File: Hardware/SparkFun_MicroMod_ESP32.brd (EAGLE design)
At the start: 22 x 22 mm, 53 parts, among them J1 MICROMOD-2222, Q2 MBT3904DW1T1, U1 W25QXX128MBIT-6X5, U2 ESP3212, U4 CP2102N, Y1 40MHZ, Y2 32.768kHz

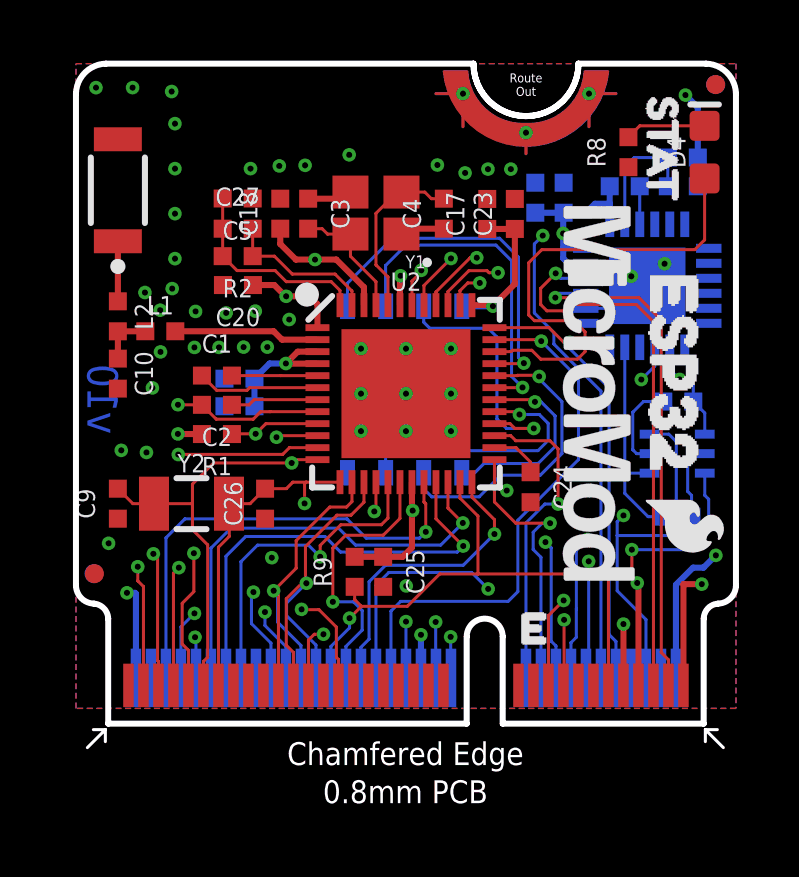
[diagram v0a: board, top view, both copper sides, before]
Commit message: Update SparkFun_MicroMod_ESP32.brd
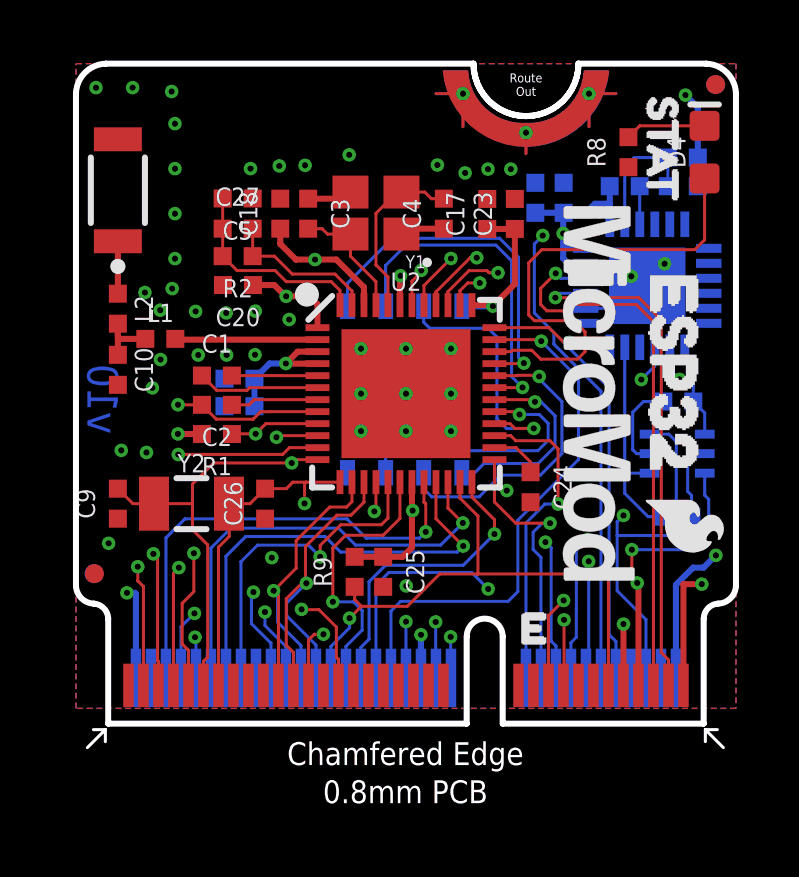
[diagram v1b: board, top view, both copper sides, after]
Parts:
- moved L2 0.25 mm to (1.40, 13.8)
- moved L1 0.25 mm to (2.81, 12.8)
- moved C10 0.13 mm to (1.40, 11.8)
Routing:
- net N$6: track 1.83 -> 2.44 mm
- net GND: vias 46 -> 45
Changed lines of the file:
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@@
 <?xml version="1.0" encoding="utf-8"?>
 <!DOCTYPE eagle SYSTEM "eagle.dtd">
-<eagle version="9.4.1">
+<eagle version="9.6.0">
 <drawing>
 <settings>
@@
 <setting verticaltext="up"/>
 </settings>
-<grid distance="0.05" unitdist="inch" unit="mm" style="lines" multiple="1" display="yes" altdistance="0.005" altunitdist="inch" altunit="inch"/>
+<grid distance="0.05" unitdist="inch" unit="inch" style="lines" multiple="1" display="yes" altdistance="0.005" altunitdist="inch" altunit="inch"/>
 <layers>
 <layer number="1" name="Top" color="4" fill="1" visible="yes" active="yes"/>
@@
 <layer number="38" name="bTest" color="7" fill="1" visible="no" active="yes"/>
 <layer number="39" name="tKeepout" color="4" fill="11" visible="yes" active="yes"/>
-<layer number="40" name="bKeepout" color="1" fill="11" visible="yes" active="yes"/>
+<layer number="40" name="bKeepout" color="1" fill="11" visible="no" active="yes"/>
 <layer number="41" name="tRestrict" color="4" fill="10" visible="no" active="yes"/>
 <layer number="42" name="bRestrict" color="1" fill="10" visible="no" active="yes"/>
 <layer number="43" name="vRestrict" color="2" fill="10" visible="no" active="yes"/>
 <layer number="44" name="Drills" color="7" fill="1" visible="no" active="yes"/>
-<layer number="45" name="Holes" color="7" fill="1" visible="no" active="yes"/>
+<layer number="45" name="Holes" color="7" fill="1" visible="yes" active="yes"/>
 <layer number="46" name="Milling" color="3" fill="1" visible="no" active="yes"/>
 <layer number="47" name="Measures" color="7" fill="1" visible="no" active="yes"/>
@@
 <layer number="50" name="dxf" color="7" fill="1" visible="no" active="yes"/>
 <layer number="51" name="tDocu" color="6" fill="1" visible="yes" active="yes"/>
-<layer number="52" name="bDocu" color="7" fill="1" visible="yes" active="yes"/>
+<layer number="52" name="bDocu" color="7" fill="1" visible="no" active="yes"/>
 <layer number="91" name="Nets" color="2" fill="1" visible="no" active="no"/>
 <layer number="92" name="Busses" color="1" fill="1" visible="no" active="no"/>
@@
 <layer number="95" name="Names" color="7" fill="1" visible="no" active="no"/>
 <layer number="96" name="Values" color="7" fill="1" visible="no" active="no"/>
-<layer number="2" name="Horz/PWR" color="16" fill="1" visible="yes" active="yes"/>
+<layer number="2" name="Horz/PWR" color="16" fill="1" visible="no" active="yes"/>
 <layer number="3" name="Route3" color="17" fill="1" visible="no" active="no"/>
 <layer number="4" name="Route4" color="18" fill="1" visible="no" active="no"/>
@@
 <layer number="13" name="Route13" color="21" fill="1" visible="no" active="no"/>
 <layer number="14" name="Route14" color="22" fill="1" visible="no" active="no"/>
-<layer number="15" name="VIRT/GND" color="23" fill="1" visible="yes" active="yes"/>
+<layer number="15" name="VIRT/GND" color="23" fill="1" visible="no" active="yes"/>
 <layer number="53" name="tGND_GNDA" color="7" fill="9" visible="no" active="no"/>
 <layer number="54" name="bGND_GNDA" color="1" fill="9" visible="no" active="no"/>
@@
 <attribute name="VALUE" x="7.781" y="11.137" size="0.762" layer="28" rot="MR90" align="center"/>
 </element>
-<element name="L1" library="SparkFun-Coils" package="0402-TIGHT" value="2.7nH" x="2.812" y="13.08" smashed="yes">
-<attribute name="NAME" x="2.812" y="13.642" size="0.6096" layer="25" font="vector" ratio="20" align="bottom-center"/>
-<attribute name="PROD_ID" value="NDUC-14236" x="2.812" y="13.08" size="1.778" layer="27" font="vector" ratio="15" display="off"/>
-<attribute name="VALUE" x="2.812" y="12.518" size="0.6096" layer="27" font="vector" ratio="20" align="top-center"/>
-</element>
-<element name="L2" library="SparkFun-Coils" package="0402-TIGHT" value="2nH" x="1.397" y="13.578" smashed="yes" rot="R270">
-<attribute name="NAME" x="1.959" y="13.578" size="0.6096" layer="25" font="vector" ratio="20" rot="R270" align="bottom-center"/>
-<attribute name="PROD_ID" value="NDUC-14238" x="1.397" y="13.578" size="1.778" layer="27" font="vector" ratio="15" rot="R270" display="off"/>
-<attribute name="VALUE" x="0.835" y="13.578" size="0.6096" layer="27" font="vector" ratio="20" rot="R270" align="top-center"/>
-</element>
-<element name="C10" library="SparkFun-Capacitors" package="0402-TIGHT" value="0.5pF" x="1.397" y="11.667" smashed="yes" rot="R270">
-<attribute name="NAME" x="1.959" y="11.667" size="0.6096" layer="25" font="vector" ratio="20" rot="R270" align="bottom-center"/>
-<attribute name="PROD_ID" value="CAP-14362" x="1.397" y="11.667" size="1.778" layer="27" font="vector" ratio="15" rot="R270" display="off"/>
-<attribute name="VALUE" x="0.835" y="11.667" size="0.6096" layer="27" font="vector" ratio="20" rot="R270" align="top-center"/>
+<element name="L1" library="SparkFun-Coils" package="0402-TIGHT" value="2.7nH" x="2.812" y="12.826" smashed="yes">
+<attribute name="NAME" x="2.812" y="13.388" size="0.6096" layer="25" font="vector" ratio="20" align="bottom-center"/>
+<attribute name="PROD_ID" value="NDUC-14236" x="2.812" y="12.826" size="1.778" layer="27" font="vector" ratio="15" display="off"/>
+<attribute name="VALUE" x="2.812" y="12.264" size="0.6096" layer="27" font="vector" ratio="20" align="top-center"/>
+</element>
+<element name="L2" library="SparkFun-Coils" package="0402-TIGHT" value="2nH" x="1.397" y="13.832" smashed="yes" rot="R270">
+<attribute name="NAME" x="1.959" y="13.832" size="0.6096" layer="25" font="vector" ratio="20" rot="R270" align="bottom-center"/>
+<attribute name="PROD_ID" value="NDUC-14238" x="1.397" y="13.832" size="1.778" layer="27" font="vector" ratio="15" rot="R270" display="off"/>
+<attribute name="VALUE" x="0.835" y="13.832" size="0.6096" layer="27" font="vector" ratio="20" rot="R270" align="top-center"/>
+</element>
+<element name="C10" library="SparkFun-Capacitors" package="0402-TIGHT" value="0.5pF" x="1.397" y="11.794" smashed="yes" rot="R270">
+<attribute name="NAME" x="1.959" y="11.794" size="0.6096" layer="25" font="vector" ratio="20" rot="R270" align="bottom-center"/>
+<attribute name="PROD_ID" value="CAP-14362" x="1.397" y="11.794" size="1.778" layer="27" font="vector" ratio="15" rot="R270" display="off"/>
+<attribute name="VALUE" x="0.835" y="11.794" size="0.6096" layer="27" font="vector" ratio="20" rot="R270" align="top-center"/>
 </element>
 <element name="FD1" library="SparkFun-Aesthetics" package="FIDUCIAL-MICRO" value="FIDUCIALUFIDUCIAL" x="0.614" y="5" smashed="yes"/>
@@
 <via x="5.978" y="13.751" extent="1-16" drill="0.2"/>
 <via x="7.108" y="13.471" extent="1-16" drill="0.2"/>
-<via x="2.818" y="12.391" extent="1-16" drill="0.2"/>
+<via x="2.818" y="12.137" extent="1-16" drill="0.2"/>
 <via x="1.088" y="6.011" extent="1-16" drill="0.2"/>
-<via x="6.378" y="12.551" extent="1-16" drill="0.2"/>
 <wire x1="9.15" y1="17.718" x2="8.93" y2="17.498" width="0.2032" layer="1"/>
 <wire x1="8.93" y1="17.498" x2="7.74" y2="17.498" width="0.2032" layer="1"/>
@@
 <via x="3.988" y="13.741" extent="1-16" drill="0.2"/>
 <via x="5.008" y="13.691" extent="1-16" drill="0.2"/>
-<via x="5.588" y="12.551" extent="1-16" drill="0.2"/>
-<via x="4.768" y="12.541" extent="1-16" drill="0.2"/>
-<via x="3.948" y="12.541" extent="1-16" drill="0.2"/>
+<via x="5.969" y="12.297" extent="1-16" drill="0.2"/>
+<via x="5.022" y="12.287" extent="1-16" drill="0.2"/>
+<via x="4.075" y="12.287" extent="1-16" drill="0.2"/>
 <via x="19.62" y="15.33" extent="1-16" drill="0.2"/>
 <via x="12.972" y="18.357" extent="1-16" drill="0.2"/>
@@
 <contactref element="L2" pad="1"/>
 <contactref element="A1" pad="FEED"/>
-<wire x1="1.397" y1="14.078" x2="1.397" y2="16.08" width="0.2032" layer="1"/>
+<wire x1="1.397" y1="14.332" x2="1.397" y2="16.08" width="0.2032" layer="1"/>
 </signal>
 <signal name="N$6">
@@
 <contactref element="L1" pad="1"/>
 <contactref element="C10" pad="1"/>
-<wire x1="2.312" y1="13.08" x2="2.31" y2="13.078" width="0.2032" layer="1"/>
-<wire x1="2.31" y1="13.078" x2="1.397" y2="13.078" width="0.2032" layer="1"/>
-<wire x1="1.397" y1="12.167" x2="1.397" y2="13.078" width="0.2032" layer="1"/>
+<wire x1="2.312" y1="12.826" x2="1.423" y2="12.826" width="0.2032" layer="1"/>
+<wire x1="1.423" y1="12.826" x2="1.397" y2="12.852" width="0.2032" layer="1"/>
+<wire x1="1.397" y1="13.332" x2="1.397" y2="12.852" width="0.2032" layer="1"/>
+<wire x1="1.397" y1="12.294" x2="1.397" y2="13.332" width="0.2032" layer="1"/>
 </signal>
 <signal name="N$8">
 <contactref element="U2" pad="2"/>
 <contactref element="L1" pad="2"/>
-<wire x1="6.87" y1="12.8" x2="8.05" y2="12.8" width="0.2032" layer="1"/>
-<wire x1="3.312" y1="13.08" x2="6.59" y2="13.08" width="0.2032" layer="1"/>
-<wire x1="6.59" y1="13.08" x2="6.87" y2="12.8" width="0.2032" layer="1"/>
+<wire x1="8.05" y1="12.8" x2="3.455" y2="12.8" width="0.2032" layer="1"/>
+<wire x1="3.455" y1="12.8" x2="3.429" y2="12.826" width="0.2032" layer="1"/>
+<wire x1="3.312" y1="12.826" x2="3.429" y2="12.826" width="0.2032" layer="1"/>
 </signal>
 </signals>

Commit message: Updated design
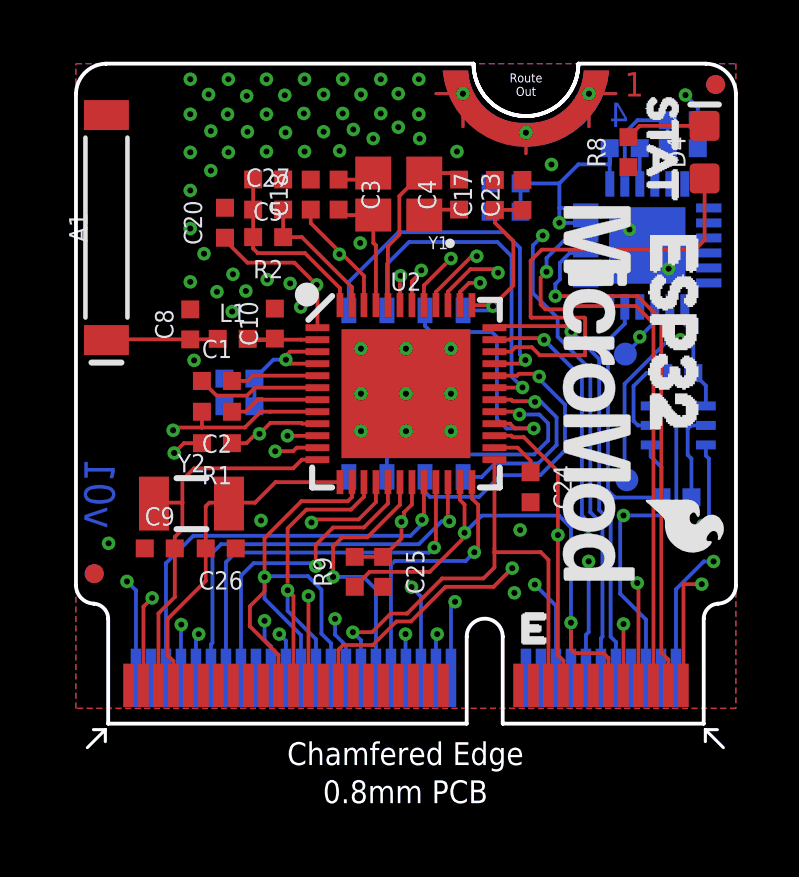
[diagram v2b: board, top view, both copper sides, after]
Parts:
- removed L2: 2nH, SparkFun-Coils:0402-TIGHT
- added C8: (no value), SparkFun-Capacitors:0402-TIGHT
- added TP1, TP2: (no value), SparkFun-Connectors:PAD.03X.03
- A1: device SparkFun-RF:ANT-2.4GHZ-3.2X1.6X1.2MM-REDUCED_KEEPOUT -> SparkFun-RF:ANT-2.4GHZ-8.0X1.0MM
- C10: value 0.5pF -> (none)
- Q2: device esp32-thing-temp:SC70-6 -> SparkFun-DiscreteSemi:SC70-6
- U2: value ESP3212 -> ESP32; device esp32-thing-temp:QFN48-0.4MM -> SparkFun-RF:QFN48-0.4MM
- Y1: value 40MHZ -> 40MHz
- moved C10 5.45 mm to (6.63, 13.3), turned to 90 degrees
- moved LOGO3 4.02 mm to (18.6, 5.92)
- moved L1 2.41 mm to (5.22, 12.8)
- moved C20 2.12 mm to (4.97, 16.7), turned to 90 degrees
- moved C26 2.10 mm to (4.83, 5.84), turned to 180 degrees
- moved LOGO2 2.07 mm to (7.11, 17.3)
- moved C9 2.04 mm to (2.79, 5.84), turned to 0 degrees
- moved C7 1.99 mm to (14.3, 18.0), turned to 0 degrees
- moved U4 1.35 mm to (19.0, 15.9)
- moved U$3 1.35 mm to (19.9, 17.7)
- moved A1 1.30 mm to (1.02, 16.5)
- moved R4 1.27 mm to (20.2, 19.2)
- moved R5 1.27 mm to (18.3, 19.2)
- moved R3 1.24 mm to (20.2, 20.1)
- moved C18 1.20 mm to (7.83, 17.6)
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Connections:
- net 13 renamed 13-SPI_!CS!/SD_DATA3
- net 14 renamed 14-SPI_SCK/SD_CLK
- net 15 renamed 15-SPI_MOSI/SD_CMD
- net 2 renamed 2-SPI_MISO/SD_DATA0
- net 21 renamed 21-SDA
- net 22 renamed 22-SCL
- net 23 renamed 23-D0
- net 27 renamed 27-D1
- net 34 renamed 34-A0
- net 35 renamed 35-A1
- net 39 renamed 39-BATT/3
- net 5 renamed 5-STAT_LED
- net CHIP_PU renamed !RESET
- net FLASH_SCK renamed FLASH_SD_CLK
- net FLASH_SCS renamed FLASH_SD_CMD
- net FLASH_SDI renamed FLASH_SD_DATA1
- net FLASH_SDO renamed FLASH_SD_DATA0
- net FLASH_SHD renamed FLASH_SD_DATA2
- net FLASH_SWP renamed FLASH_SD_DATA3
- removed net 0: J1.11, J1.48, Q2.6, R9.1, U2.23
- removed net 12: J1.46, J1.68, U2.18
- removed net 16: J1.20, J1.54, J1.73, U2.25
- removed net 17: J1.22, J1.56, J1.71, U2.27
- removed net 18: J1.40, U2.35
- removed net 19: J1.16, J1.42, U2.38
- removed net 25: J1.52, J1.55, J1.69, U2.14
- removed net 26: J1.50, J1.53, J1.67, U2.15
- removed net 32K_XN: C26.2, J1.47, J1.63, U2.13, Y2.P$2
- removed net 32K_XP: C9.2, J1.32, J1.65, U2.12, Y2.P$1
- removed net 4: J1.44, J1.66, U2.24
- removed net N$6: C10.1, L1.1, L2.2
- removed net V_RTC: J1.72
- new net 0-!BOOT!/I2C_!INT: J1.11, J1.16, Q2.6, R9.1, U2.23
- new net 12-SD_DATA2/G1: J1.42, J1.68, U2.18
- new net 16-G2/RX1/AUD_IN: J1.19, J1.44, J1.54, U2.25
- new net 17-G3/TX1/AUD_OUT: J1.17, J1.46, J1.56, U2.27
- new net 18-PWM0: J1.32, U2.35
- new net 19-PWM1: J1.47, U2.38
- new net 25-G4/AUD_LRCLK/SCL1: J1.48, J1.52, J1.55, U2.14
- new net 26-G5/AUD_BCLK/SDA1: J1.50, J1.53, J1.73, U2.15
- new net 32-G6/RTC: C9.2, J1.71, U2.12, Y2.P$1
- new net 33-G7/RTC: C26.2, J1.69, U2.13, Y2.P$2
- new net 4-SD_DATA1/G0: J1.40, J1.66, U2.24
- net GND: now also C8.2
- net N$5: now also C8.1, L1.1; no longer L2.1
- net N$8: now also C10.1
- net U0RXD: now also TP1.P$1; no longer J1.19
- net U0TXD: now also TP2.P$1; no longer J1.17
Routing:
- net 17: track 40.9 -> 0.00 mm, vias 4 -> 0
- net 16: track 40.6 -> 0.00 mm, vias 4 -> 0
- net 19: track 29.9 -> 0.00 mm, vias 3 -> 0
- net 0-!BOOT!/I2C_!INT: track 0.00 -> 26.9 mm, vias 0 -> 3
- net 0: track 25.5 -> 0.00 mm, vias 2 -> 0
- net 17-G3/TX1/AUD_OUT: track 0.00 -> 25.5 mm, vias 0 -> 3
- net 32K_XP: track 25.3 -> 0.00 mm, vias 2 -> 0
- net 4: track 24.5 -> 0.00 mm, vias 2 -> 0
- net 19-PWM1: track 0.00 -> 24.0 mm, vias 0 -> 2
- net 26-G5/AUD_BCLK/SDA1: track 0.00 -> 23.0 mm, vias 0 -> 2
- net 4-SD_DATA1/G0: track 0.00 -> 22.6 mm, vias 0 -> 2
- net 26: track 21.0 -> 0.00 mm, vias 2 -> 0
- net 16-G2/RX1/AUD_IN: track 0.00 -> 21.0 mm, vias 0 -> 2
- net 12-SD_DATA2/G1: track 0.00 -> 19.4 mm, vias 0 -> 2
- net 25: track 19.0 -> 0.00 mm, vias 2 -> 0
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- added copper zone on layer 15, net 3.3V
- added copper zone on layer 2, net GND
- removed copper zone on layer 2, net 3.3V
- removed copper zone on layer 15, net GND
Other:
- board text added: "1"
- board text added: "2"
- board text added: "3"
- board text added: "4"
- board text added: "v01"
- board text removed: "v10"
